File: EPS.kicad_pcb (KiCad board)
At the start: 4 copper layers, 90.2 x 95.9 mm, 197 parts, among them IC1 BQ7791514PWR, IC10 INA260AIPWR, IC12 LM74700QDBVRQ1, IC13 LM74700QDBVRQ1, IC14 LM5176PWPR, IC15 SN65HVD1782QDRQ1, IC16 TPS2121RUXR, IC17 TCAN1046AVDRQ1, IC18 INA260AIPWR, IC19 LM5060Q1MM_NOPB, IC2 INA260AIPWR, IC20 LM5060Q1MM_NOPB, IC21 MCP2517FD-H_SL, IC3 INA260AIPWR, IC4 INA260AIPWR, IC5 TPS22990DMLR, IC6 TPS22990DMLR, IC7 TPS22990DMLR, IC9 INA260AIPWR, J1 Barrel_Jack_Switch, J2 PH1RA-02-UA, J3 WJ126V-5.0-2P, J4 USB_C_Receptacle_USB2.0_16P, J6 TagConnect_TC2030-NL, Q10 BSZ067N06LS3_G, Q11 BSZ067N06LS3_G, Q12 BSZ067N06LS3_G, Q13 BSZ067N06LS3_G, Q15 BSZ067N06LS3_G, Q16 BSZ067N06LS3_G, Q5 BSZ067N06LS3_G, Q6 BSZ067N06LS3_G, Q8 BSZ067N06LS3_G, Q9 BSZ067N06LS3_G, U2 RP2354A_60QFN, Y1 ABM8AIG-20MHz-12-2Z-T3, Y2 ABM8-272-T3

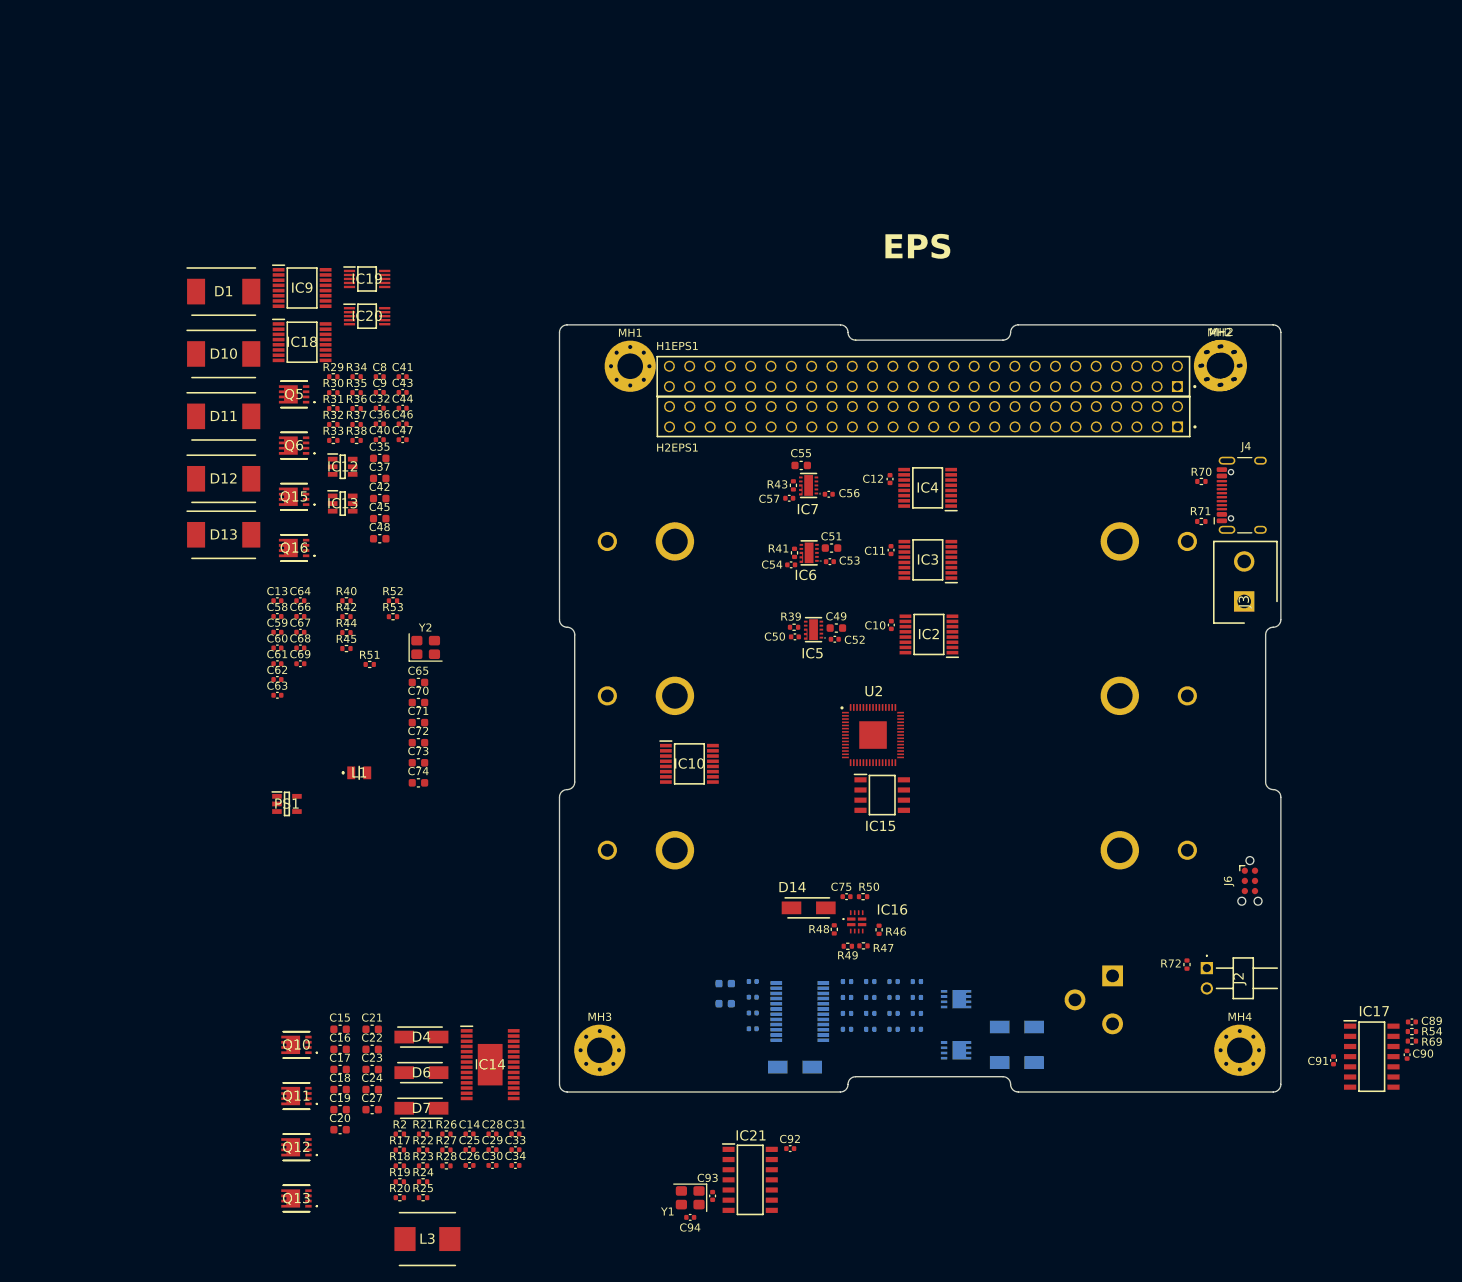
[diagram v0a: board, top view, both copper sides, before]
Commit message: Initial layout completed
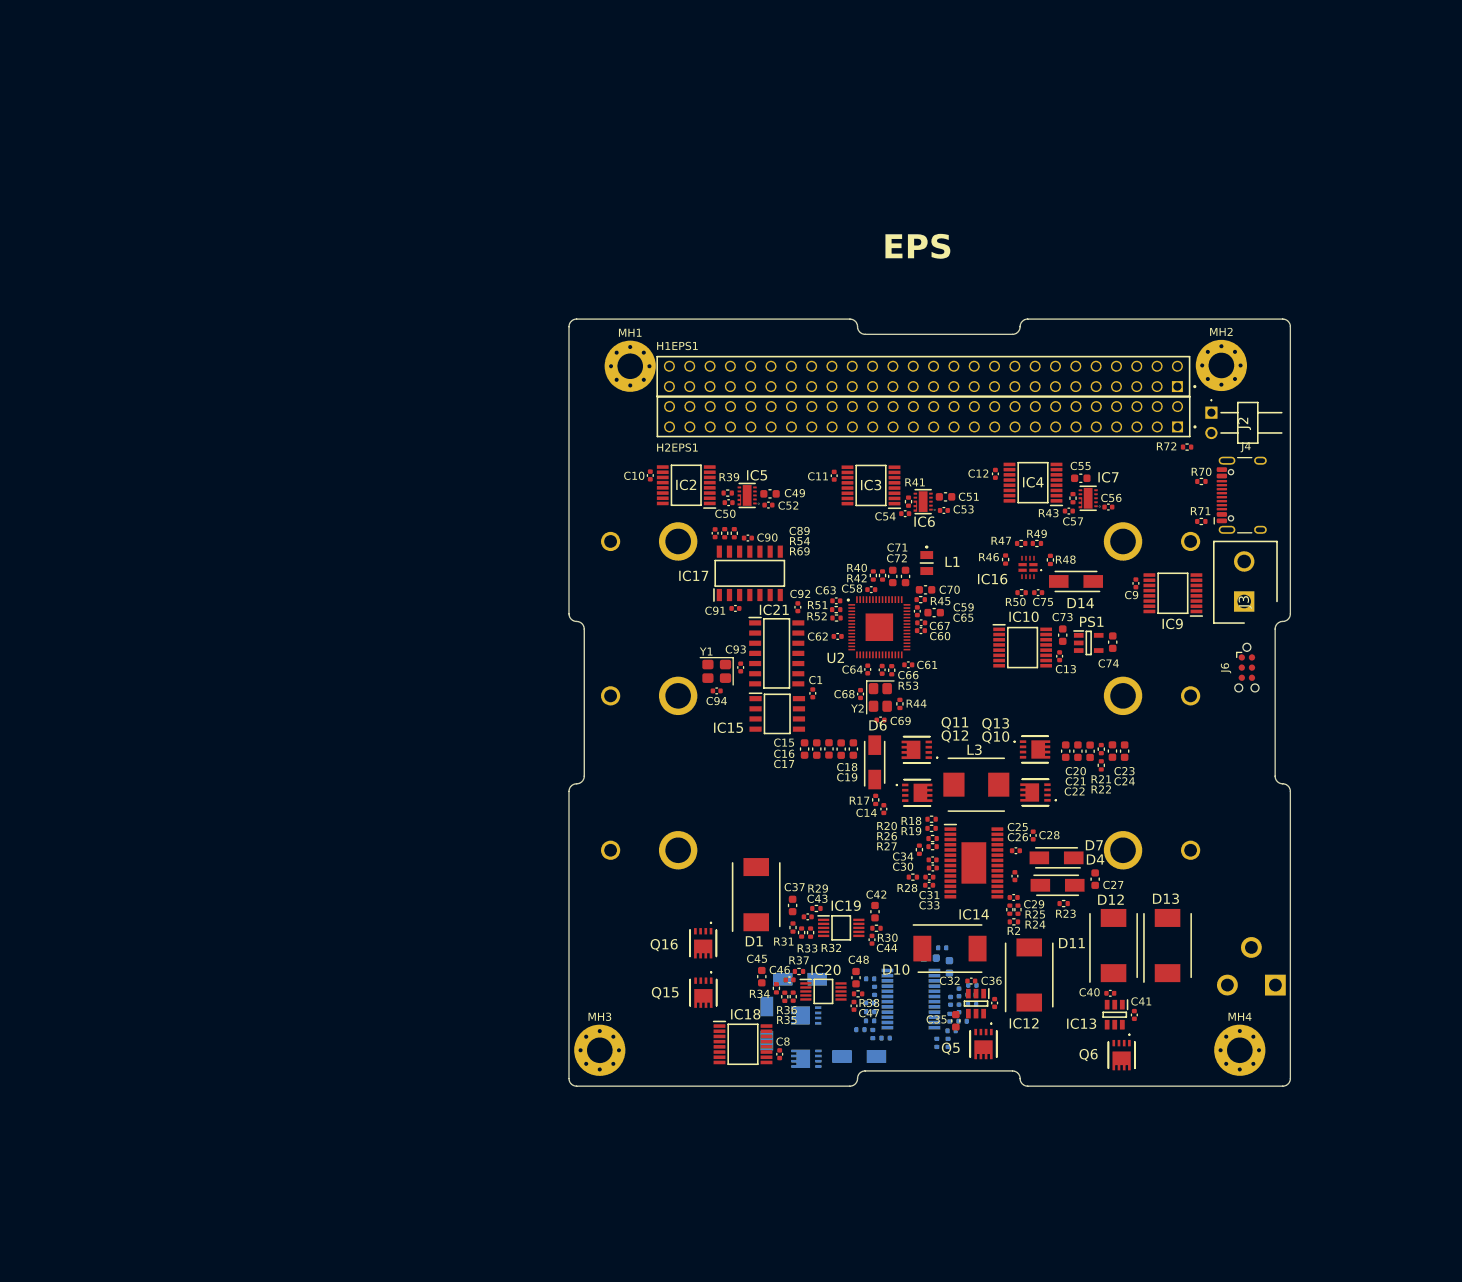
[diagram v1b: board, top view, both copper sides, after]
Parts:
- removed the MH2 at (258.9, 96.5)
- added C1: 100n, Capacitor_SMD:C_0402_1005Metric, F.Cu at (208.0, 137.4)
- D4, D7: value 40V 2A -> CDBA240LL-HF, 40V 2A
- moved D13 128.7 mm to (252.4, 168.9), turned to 90 degrees
- moved Q6 128.5 mm to (246.6, 182.6), turned to 90 degrees
- moved D12 125.6 mm to (245.6, 168.9), turned to 90 degrees
- moved D11 122.5 mm to (235.1, 172.6), turned to 90 degrees
- moved C41 121.4 mm to (248.2, 177.6), turned to 90 degrees
- moved Q5 118.4 mm to (229.4, 181.2), turned to 90 degrees
- moved D10 117.3 mm to (225.2, 169.3)
- moved IC13 115.7 mm to (245.8, 177.6), turned to -90 degrees
- moved IC9 115.3 mm to (253.0, 124.9), turned to 180 degrees
- moved C40 114.6 mm to (245.2, 174.9)
- moved Q13 108.0 mm to (235.8, 144.4), turned to 180 degrees
- moved C89 106.4 mm to (195.8, 117.4), turned to -90 degrees
- moved R54 106.1 mm to (197.0, 117.4), turned to 90 degrees
- moved R69 105.9 mm to (198.2, 117.4), turned to -90 degrees
- moved C36 105.6 mm to (230.8, 176.1), turned to 90 degrees
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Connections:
- BT1 pad 1+: +BATT -> /Batteries/VC1
- BT1 pad 1-: +BATT -> GND
- BT1 pad 2+: +BATT -> /Batteries/VC2
- BT1 pad 2-: +BATT -> /Batteries/VC1
- BT1 pad 3-: +BATT -> /Batteries/VC2
- C10 pad 2: +BATT -> GND
- C11 pad 2: +BATT -> GND
- C12 pad 2: +BATT -> GND
- C13 pad 2: +BATT -> GND
- C14 pad 2: +BATT -> GND
- C15 pad 2: +BATT -> GND
- C16 pad 2: +BATT -> GND
- C17 pad 2: +BATT -> GND
- C18 pad 2: +BATT -> GND
- C19 pad 2: +BATT -> GND
- C2 pad 2: +BATT -> GND
- C20 pad 2: +BATT -> GND
- C21 pad 2: +BATT -> GND
- C22 pad 2: +BATT -> GND
- C23 pad 2: +BATT -> GND
- C24 pad 2: +BATT -> GND
- C25 pad 2: +BATT -> GND
- C27 pad 2: +BATT -> GND
- C3 pad 1: +BATT -> GND
- C30 pad 2: +BATT -> GND
- C32 pad 2: +BATT -> GND
- C33 pad 2: +BATT -> GND
- C34 pad 2: +BATT -> GND
- C35 pad 2: +BATT -> GND
- C37 pad 2: +BATT -> GND
- C40 pad 2: +BATT -> GND
- C42 pad 2: +BATT -> GND
- C43 pad 2: +BATT -> GND
- C44 pad 2: +BATT -> GND
- C45 pad 2: +BATT -> GND
- C46 pad 2: +BATT -> GND
- C47 pad 2: +BATT -> GND
- C48 pad 2: +BATT -> GND
- C49 pad 2: +BATT -> GND
- C50 pad 2: +BATT -> GND
- C51 pad 2: +BATT -> GND
- C52 pad 2: +BATT -> GND
- C53 pad 2: +BATT -> GND
- C54 pad 2: +BATT -> GND
- C55 pad 2: +BATT -> GND
- C56 pad 2: +BATT -> GND
- C57 pad 2: +BATT -> GND
- C58 pad 2: +BATT -> GND
- C59 pad 2: +BATT -> GND
- C6 pad 2: +BATT -> GND
- C60 pad 2: +BATT -> GND
- C61 pad 2: +BATT -> GND
- C62 pad 2: +BATT -> GND
- C63 pad 2: +BATT -> GND
- C64 pad 2: +BATT -> GND
- C65 pad 2: +BATT -> GND
- C66 pad 2: +BATT -> GND
- C67 pad 2: +BATT -> GND
- C68 pad 1: +BATT -> GND
- C69 pad 1: +BATT -> GND
- C7 pad 1: +BATT -> GND
- C70 pad 2: +BATT -> GND
- C71 pad 2: +BATT -> GND
- C72 pad 2: +BATT -> GND
- C73 pad 2: +BATT -> GND
- C74 pad 2: +BATT -> GND
- C75 pad 2: +BATT -> GND
- C8 pad 2: +BATT -> GND
- C89 pad 2: +BATT -> GND
- C9 pad 2: +BATT -> GND
- C90 pad 2: +BATT -> GND
- C91 pad 2: +BATT -> GND
- C92 pad 2: +BATT -> GND
- C93 pad 1: +BATT -> GND
- C93 pad 2: Net-(IC21-OSC2) -> Net-(C93-Pad2)
- C94 pad 1: +BATT -> GND
- D1 pad 2: +BATT -> GND
- D11 pad 1: +BATT -> GND
- D13 pad 1: +BATT -> GND
- D14 pad 1: +BATT -> GND
- D3 pad 2: Net-(D3-A) -> PACK-
- H1EPS1 pad 29: +BATT -> GND
- H1EPS1 pad 30: +BATT -> GND
- H1EPS1 pad 31: +BATT -> GND
- H1EPS1 pad 32: +BATT -> GND
- H2EPS1 pad 29: +BATT -> GND
- H2EPS1 pad 30: +BATT -> GND
- H2EPS1 pad 31: +BATT -> GND
- H2EPS1 pad 32: +BATT -> GND
- IC1 pad 10: +BATT -> GND
- IC1 pad 20: +BATT -> GND
- IC1 pad 23: +BATT -> GND
- IC1 pad 24: +BATT -> GND
- IC1 pad 9: +BATT -> GND
- IC10 pad 11: +BATT -> GND
- IC10 pad 6: +BATT -> GND
- IC12 pad 2: +BATT -> GND
- IC13 pad 2: +BATT -> GND
- IC14 pad 10: +BATT -> GND
- IC14 pad 13: +BATT -> GND
- IC14 pad 14: +BATT -> GND
- IC14 pad 22: +BATT -> GND
- IC14 pad 29: +BATT -> GND
- IC14 pad 5: +BATT -> GND
- IC15 pad 5: +BATT -> GND
- IC16 pad 3: +BATT -> GND
- IC16 pad 6: +BATT -> GND
- IC16 pad 9: +BATT -> GND
- IC17 pad 14: +BATT -> GND
- IC17 pad 2: +BATT -> GND
- IC17 pad 5: +BATT -> GND
- IC18 pad 11: +BATT -> GND
- IC18 pad 4: +BATT -> GND
- IC18 pad 6: +BATT -> GND
- IC19 pad 6: +BATT -> GND
- IC2 pad 11: +BATT -> GND
- IC2 pad 4: +BATT -> GND
- IC2 pad 6: +BATT -> GND
- IC20 pad 6: +BATT -> GND
- IC21 pad 5: Net-(IC21-OSC2) -> unconnected-(IC21-OSC2-Pad5)
- IC21 pad 7: +BATT -> GND
- IC3 pad 11: +BATT -> GND
- IC3 pad 5: +BATT -> GND
- IC3 pad 6: +BATT -> GND
- IC4 pad 11: +BATT -> GND
- IC4 pad 6: +BATT -> GND
- IC5 pad 6: +BATT -> GND
- IC6 pad 6: +BATT -> GND
- IC7 pad 6: +BATT -> GND
- IC9 pad 11: +BATT -> GND
- IC9 pad 4: +BATT -> GND
- IC9 pad 6: +BATT -> GND
- J1 pad 2: +BATT -> PACK-
- J2 pad 2: +BATT -> GND
- J3 pad 2: +BATT -> GND
- J4 pad A1: +BATT -> GND
- J4 pad A12: +BATT -> GND
- J4 pad B1: +BATT -> GND
- J4 pad B12: +BATT -> GND
- J4 pad S1: +BATT -> GND
- J6 pad 5: +BATT -> GND
- MH1 pad 1: +BATT -> GND
- MH2 pad 1: +BATT -> GND
- MH3 pad 1: +BATT -> GND
- MH4 pad 1: +BATT -> GND
- PS1 pad 2: +BATT -> GND
- Q9 pad 1: Net-(D3-A) -> PACK-
- Q9 pad 2: Net-(D3-A) -> PACK-
- Q9 pad 3: Net-(D3-A) -> PACK-
- R12 pad 1: Net-(D3-A) -> PACK-
- R13 pad 1: Net-(D3-A) -> PACK-
- R14 pad 2: +BATT -> GND
- R16 pad 2: +BATT -> GND
- R19 pad 1: +BATT -> GND
- R2 pad 2: +BATT -> GND
- R22 pad 2: +BATT -> GND
- R25 pad 2: +BATT -> GND
- R26 pad 1: +BATT -> GND
- R27 pad 1: +BATT -> GND
- R28 pad 1: +BATT -> GND
- R33 pad 1: +BATT -> GND
- R36 pad 1: +BATT -> GND
- R4 pad 1: +BATT -> /Batteries/VC2
- R47 pad 2: +BATT -> GND
- R49 pad 2: +BATT -> GND
- R5 pad 1: +BATT -> /Batteries/VC1
- R50 pad 2: +BATT -> GND
- R6 pad 1: +BATT -> GND
- R7 pad 1: +BATT -> GND
- R70 pad 1: +BATT -> GND
- R71 pad 1: +BATT -> GND
- TH1 pad 2: +BATT -> GND
- U2 pad 1: +BATT -> 3V3
- U2 pad 11: +BATT -> 3V3
- U2 pad 20: +BATT -> 3V3
- U2 pad 23: +BATT -> 1V1
- U2 pad 30: +BATT -> 3V3
- U2 pad 38: +BATT -> 3V3
- U2 pad 39: +BATT -> 1V1
- U2 pad 44: +BATT -> 3V3
- U2 pad 45: +BATT -> 3V3
- U2 pad 47: +BATT -> GND
- U2 pad 53: +BATT -> 3V3
- U2 pad 54: +BATT -> 3V3
- U2 pad 6: +BATT -> 1V1
- U2 pad 61: +BATT -> GND
- Y1 pad 1: Net-(IC21-OSC2) -> Net-(C93-Pad2)
- Y1 pad 2: +BATT -> GND
- Y1 pad 4: +BATT -> GND
- Y2 pad 2: +BATT -> GND
- Y2 pad 4: +BATT -> GND
